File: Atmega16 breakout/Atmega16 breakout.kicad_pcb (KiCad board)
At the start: 2 copper layers, 111.8 x 88.9 mm, 50 parts, among them IC1 AZ1117-3.3, IC2 AZ1117-5.0, IC5 NLV17SZ17DFT2G, IC7 ATmega16A-P, J1 Barrel_Jack_Switch, J10 Conn_01x05, J11 Conn_01x05, J12 Conn_01x05, J13 AVCC Jumper, J14 Conn_01x40, J15 Conn_01x40, J16 LED buffer bypass, J2 ISP, J3 JTAG, J4 Vcc Select, J5 FTDI power, J6 FTDI connector, J7 Conn_01x05, J8 Conn_01x05, J9 Conn_01x05, SW1 Reset, X2 16 MHz

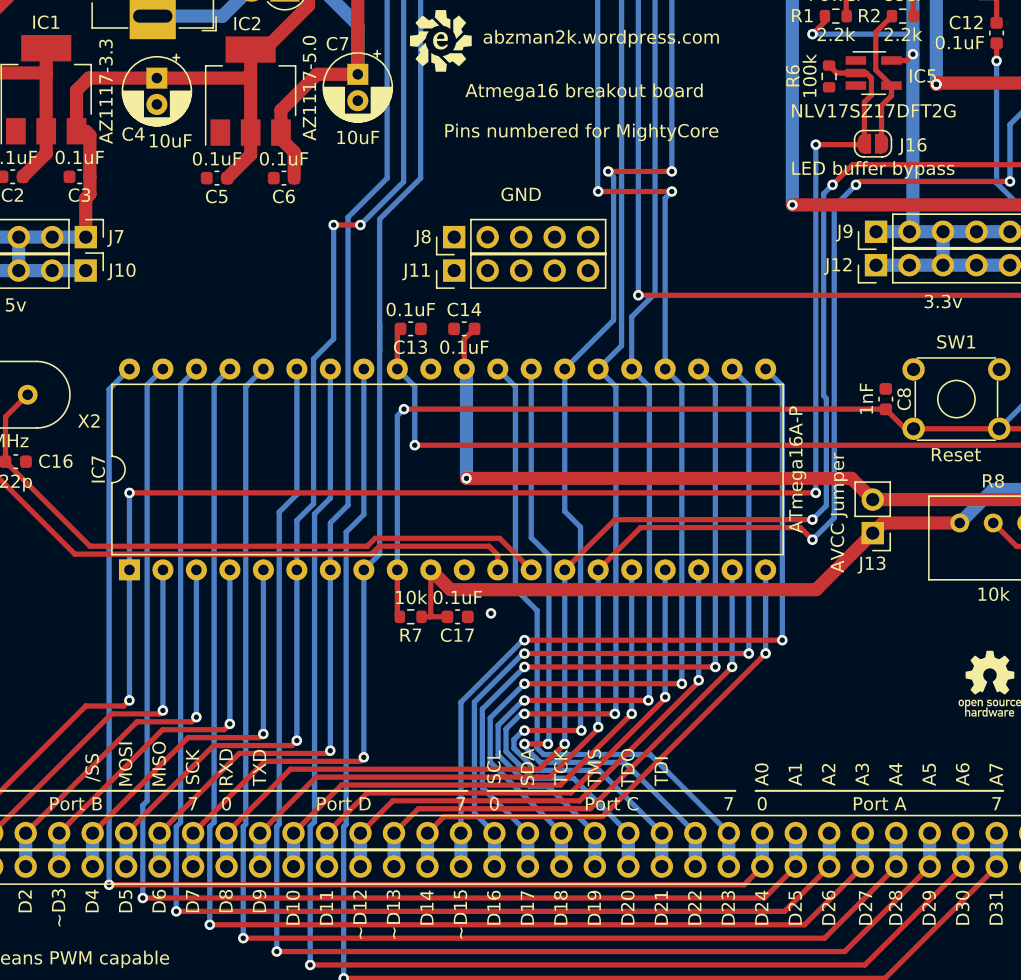
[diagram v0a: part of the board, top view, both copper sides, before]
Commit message: added gerbers, fixed ERC/DRC
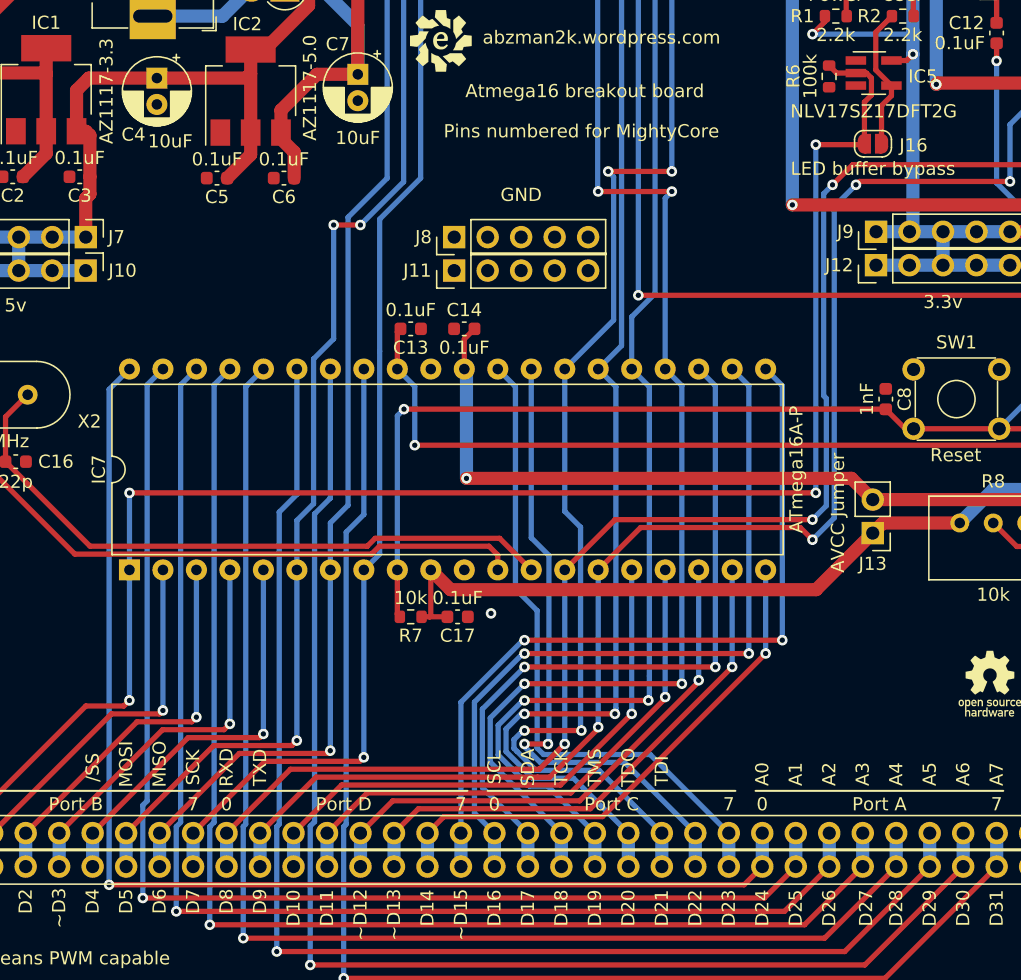
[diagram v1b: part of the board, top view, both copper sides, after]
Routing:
- net PB7: track 85.7 -> 83.5 mm
- net PA2: track 96.3 -> 95.3 mm
- net VCC: vias 2 -> 1
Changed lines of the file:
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@@
       (layerselection 0x00010fc_ffffffff)
       (disableapertmacros false)
-      (usegerberextensions false)
-      (usegerberattributes true)
-      (usegerberadvancedattributes true)
-      (creategerberjobfile true)
+      (usegerberextensions true)
+      (usegerberattributes false)
+      (usegerberadvancedattributes false)
+      (creategerberjobfile false)
       (svguseinch false)
       (svgprecision 6)
@@
       (plotinvisibletext false)
       (sketchpadsonfab false)
-      (subtractmaskfromsilk false)
+      (subtractmaskfromsilk true)
       (outputformat 1)
       (mirror false)
-      (drillshape 1)
+      (drillshape 0)
       (scaleselection 1)
-      (outputdirectory "")
+      (outputdirectory "atmega 16 breakout gerbers/")
     )
   )
@@
   (segment (start 78.962 58.96) (end 79.3015 58.6205) (width 1) (layer "F.Cu") (net 3))
   (segment (start 67.024 58.96) (end 66.0935 59.8905) (width 1) (layer "F.Cu") (net 3))
-  (segment (start 66.792 73.559) (end 66.787 73.564) (width 1) (layer "F.Cu") (net 3))
   (segment (start 67.1085 67.7655) (end 67.1085 66.446) (width 1) (layer "F.Cu") (net 3))
   (segment (start 66.0935 62.992) (end 66.802 62.992) (width 1) (layer "F.Cu") (net 3))
@@
   (segment (start 111.267489 45.390489) (end 112.517 46.64) (width 0.4) (layer "F.Cu") (net 8))
   (via (at 131.318 59.436) (size 0.8) (drill 0.4) (layers "F.Cu" "B.Cu") (net 8))
-  (via (at 131.318 59.436) (size 0.8) (drill 0.4) (layers "F.Cu" "B.Cu") (net 8))
   (segment (start 127 46.64) (end 128.549511 45.090489) (width 1) (layer "B.Cu") (net 8))
   (segment (start 139.91644 62.93356) (end 139.91644 90.17) (width 1) (layer "B.Cu") (net 8))
@@
   (segment (start 87.889 96.271) (end 89.088511 95.071489) (width 0.4) (layer "B.Cu") (net 28))
   (segment (start 89.088511 69.661489) (end 92.197 66.553) (width 0.4) (layer "B.Cu") (net 28))
-  (segment (start 89.088511 77.912511) (end 89.088511 77.535489) (width 0.4) (layer "B.Cu") (net 28))
   (segment (start 92.197 66.553) (end 92.197 46.64) (width 0.4) (layer "B.Cu") (net 28))
   (segment (start 74.935 118.776) (end 74.935 116.236) (width 1) (layer "B.Cu") (net 28))
   (segment (start 89.088511 79.690511) (end 89.088511 69.661489) (width 0.4) (layer "B.Cu") (net 28))
   (segment (start 87.889 110.485) (end 87.889 96.271) (width 0.4) (layer "B.Cu") (net 28))
-  (segment (start 89.088511 79.690511) (end 89.088511 77.912511) (width 0.4) (layer "B.Cu") (net 28))
   (segment (start 100.076 109.474) (end 101.854 109.474) (width 0.4) (layer "F.Cu") (net 29))
   (via (at 100.076 109.474) (size 0.8) (drill 0.4) (layers "F.Cu" "B.Cu") (net 29))
@@
   (segment (start 73.66 120.142) (end 73.66 122.174) (width 0.4) (layer "B.Cu") (net 42))
   (segment (start 123.195 118.776) (end 123.195 116.236) (width 1) (layer "B.Cu") (net 42))
-  (segment (start 73.66 120.142) (end 73.66 121.158) (width 0.4) (layer "B.Cu") (net 42))
   (segment (start 73.989489 82.230511) (end 73.989489 115.414435) (width 0.4) (layer "B.Cu") (net 42))
   (segment (start 73.989489 115.414435) (end 73.66 115.743924) (width 0.4) (layer "B.Cu") (net 42))
